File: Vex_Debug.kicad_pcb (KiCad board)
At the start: 2 copper layers, 26 x 54 mm, 31 parts, among them J1 USB_C_Receptacle_USB2.0, U1 ESP32-C3-MINI-1-N4, U2 NCP1117-3.3_SOT223, U3 ADM3493ARZ

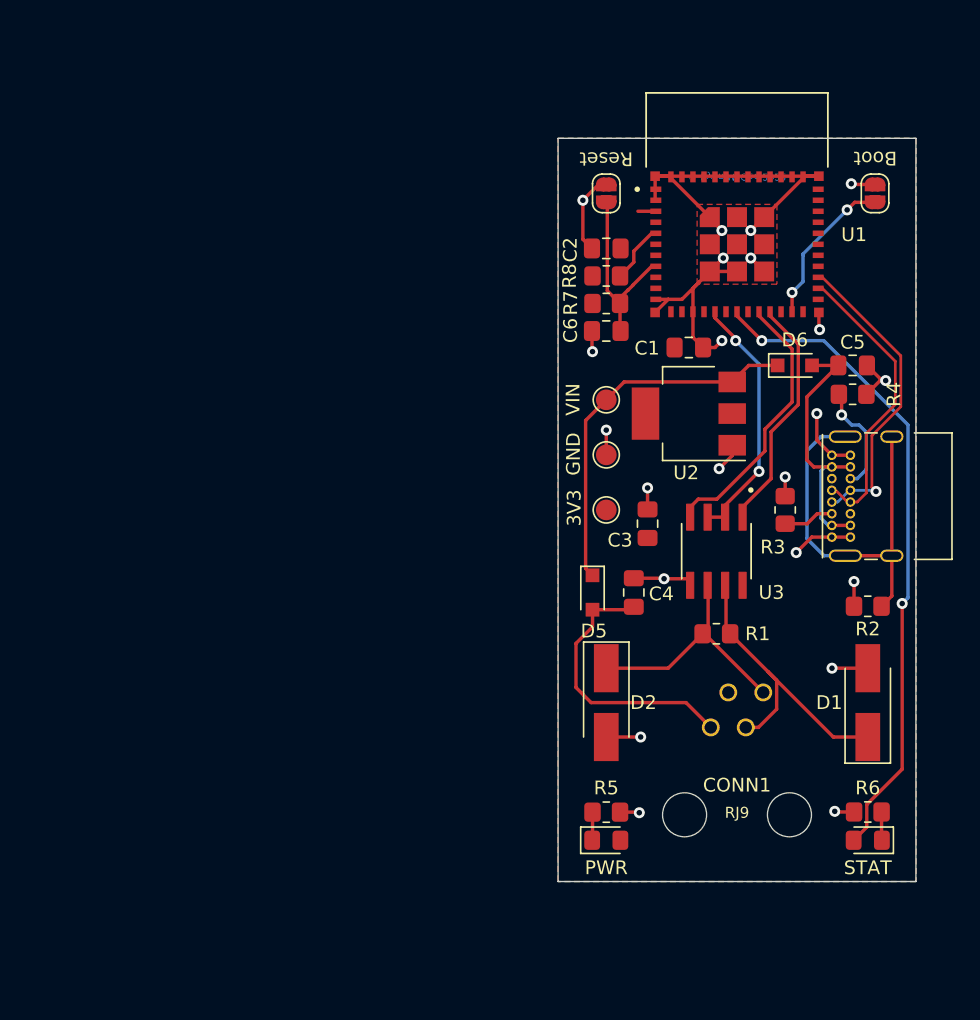
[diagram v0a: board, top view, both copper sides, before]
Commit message: Revision 2.1 release
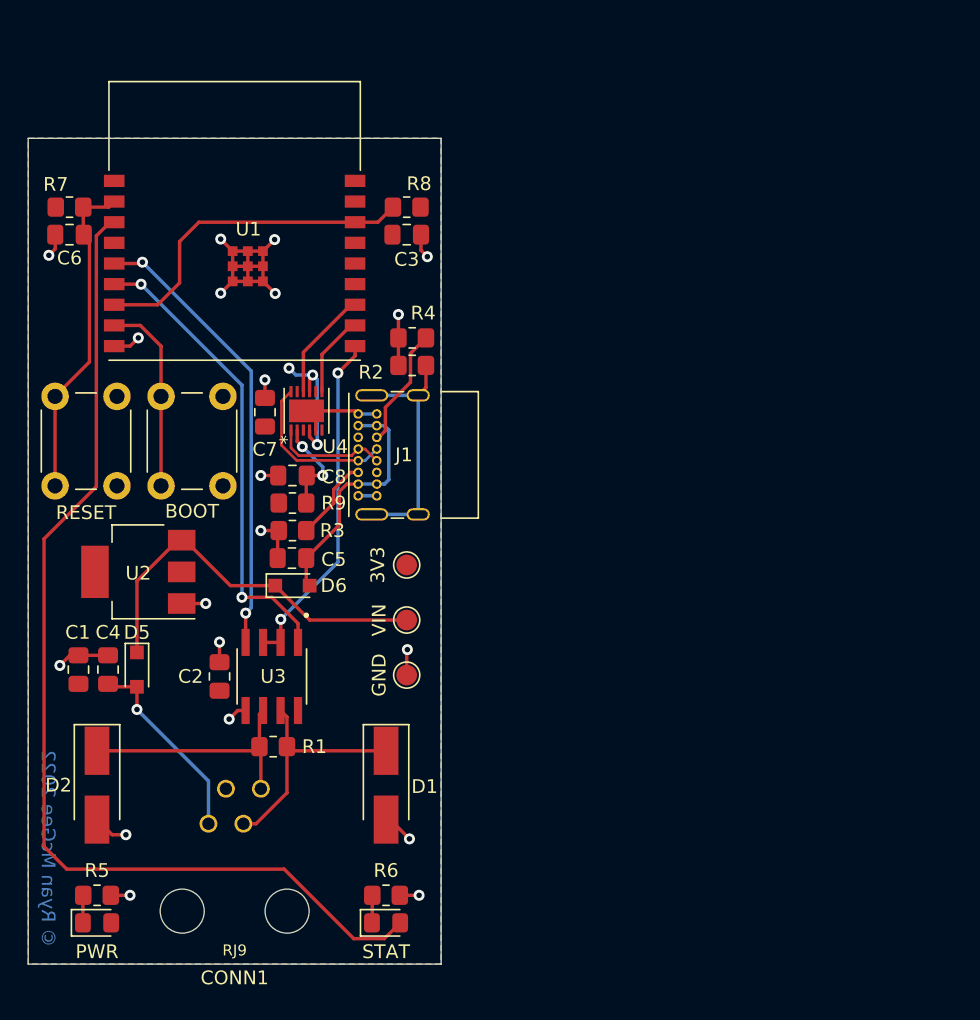
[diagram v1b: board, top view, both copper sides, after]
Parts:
- removed JP1, JP2: SolderJumper_2_Open, Jumper:SolderJumper-2_P1.3mm_Open_RoundedPad1.0x1.5mm
- added C7: 1uF, Capacitor_SMD:C_0805_2012Metric_Pad1.18x1.45mm_HandSolder, F.Cu at (97.2, 79.9)
- added C8: 1uF, Capacitor_SMD:C_0805_2012Metric_Pad1.18x1.45mm_HandSolder, F.Cu at (99.2, 84.5)
- added R9: 5.11K, Resistor_SMD:R_0805_2012Metric_Pad1.20x1.40mm_HandSolder, F.Cu at (99.2, 86.5)
- added SW1: RESET, Button_Switch_THT:SW_PUSH_6mm, F.Cu at (86.5, 78.8)
- added SW2: BOOT, Button_Switch_THT:SW_PUSH_6mm, F.Cu at (94.2, 78.8)
- added U4: FT234XD-R, USB-UART Bridge:FT234XD-R, F.Cu at (100.2, 79.8)
- R7, R8: value 10K -> 5.11K
- U1: value ESP32-C3-MINI-1-N4 -> ESP32-C3-WROOM-02-N4; footprint ESP32-C3-MINI:XCVR_ESP32-C3-MINI-1-N4 -> ESP32-C3-WROOM:ESP32-C3-WROOM-02-N4
- moved C1 50.1 mm to (83.7, 98.6), turned to 90 degrees
- moved G*** 44.7 mm to (94.2, 67.8), turned to 180 degrees
- moved C5 43.1 mm to (99.2, 90.5), turned to 180 degrees
- moved C2 41.9 mm to (93.9, 99.1), turned to 90 degrees
- moved U2 41.6 mm to (88.0, 91.5)
- moved D6 39.9 mm to (99.2, 92.5)
- moved C6 39.6 mm to (83.0, 67.0)
- moved R7 39.6 mm to (83.0, 65.0), turned to 180 degrees
- moved C4 38.6 mm to (85.8, 98.6)
- moved R5 37.5 mm to (85.0, 115.0)
- moved D2 37.5 mm to (85.0, 107.0)
- moved D3 37.5 mm to (85.0, 117.0)
- moved R2 37.4 mm to (107.9, 76.5)
- moved CONN1 37.2 mm to (95.0, 115.0)
- moved U1 36.5 mm to (95.0, 66.0)
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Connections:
- R7 pad 1: +3.3V -> Net-(C6-Pad1)
- R7 pad 2: Net-(C6-Pad1) -> +3.3V
- R8 pad 1: +3.3V -> /IO8_PULLUP
- R8 pad 2: Net-(R8-Pad2) -> +3.3V
- U1 pad 1: GND -> +3.3V
- U1 pad 10: unconnected-(U1-Pad10) -> /RS485_MODE
- U1 pad 11: GND -> /FTDI_TX
- U1 pad 12: unconnected-(U1-Pad12) -> /FTDI_RX
- U1 pad 14: GND -> unconnected-(U1-Pad14)
- U1 pad 16: /RS485_MODE -> /IO8_PULLUP
- U1 pad 18: /STAT_LED -> unconnected-(U1-Pad18)
- U1 pad 19: unconnected-(U1-Pad19) -> GND
- U1 pad 2: GND -> Net-(C6-Pad1)
- U1 pad 20: /RS485_TX -> GND
- U1 pad 21: /RS485_RX -> GND
- U1 pad 22: unconnected-(U1-Pad22) -> GND
- U1 pad 23: Net-(JP2-Pad1) -> GND
- U1 pad 24: unconnected-(U1-Pad24) -> GND
- U1 pad 25: unconnected-(U1-Pad25) -> GND
- U1 pad 26: /USB_D- -> GND
- U1 pad 27: /USB_D+ -> GND
- U1 pad 3: +3.3V -> /STAT_LED
- U1 pad 5: Net-(R8-Pad2) -> /RS485_TX
- U1 pad 6: unconnected-(U1-Pad6) -> /RS485_RX
- U1 pad 7: unconnected-(U1-Pad7) -> /IO8_PULLUP
- U1 pad 8: Net-(C6-Pad1) -> Net-(SW2-Pad2)
- U1 pad 9: unconnected-(U1-Pad9) -> GND
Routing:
- net GND: track 88.8 -> 59.4 mm, vias 22 -> 20
- net /STAT_LED: track 47.8 -> 76.8 mm, vias 2 -> 0
- net /IO8_PULLUP: track 0.00 -> 24.9 mm
- net /RS485_RX: track 17.5 -> 34.0 mm, vias 0 -> 2
- net Net-(SW2-Pad2): track 0.00 -> 14.2 mm
- net /RS485_TX: track 19.8 -> 33.2 mm, vias 0 -> 2
- net /USB_D-: track 21.0 -> 8.31 mm
- net Net-(JP2-Pad1): track 11.3 -> 0.00 mm, vias 2 -> 0
- net Net-(J1-PadS1): track 28.9 -> 17.8 mm
- net /USB_D+: track 22.8 -> 11.9 mm, vias 1 -> 0
- net Net-(C6-Pad1): track 13.7 -> 23.9 mm
- net +3.3V: track 1.30 -> 9.69 mm, vias 0 -> 3
- net /FTDI_RX: track 0.00 -> 8.04 mm
- net Net-(C8-Pad1): track 0.00 -> 7.25 mm, vias 0 -> 2
- net /RS485_MODE: track 18.5 -> 25.0 mm
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- removed copper zone on F.Cu, net GND
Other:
- board size 26 x 54 mm -> 30 x 60 mm
- board text added: "V5 Debug Board 11/27/2022 Rev 2.1"
- board text removed: "V5 Debug Board 10/23/2022 Rev 1"

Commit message: Updated to revision 3.0
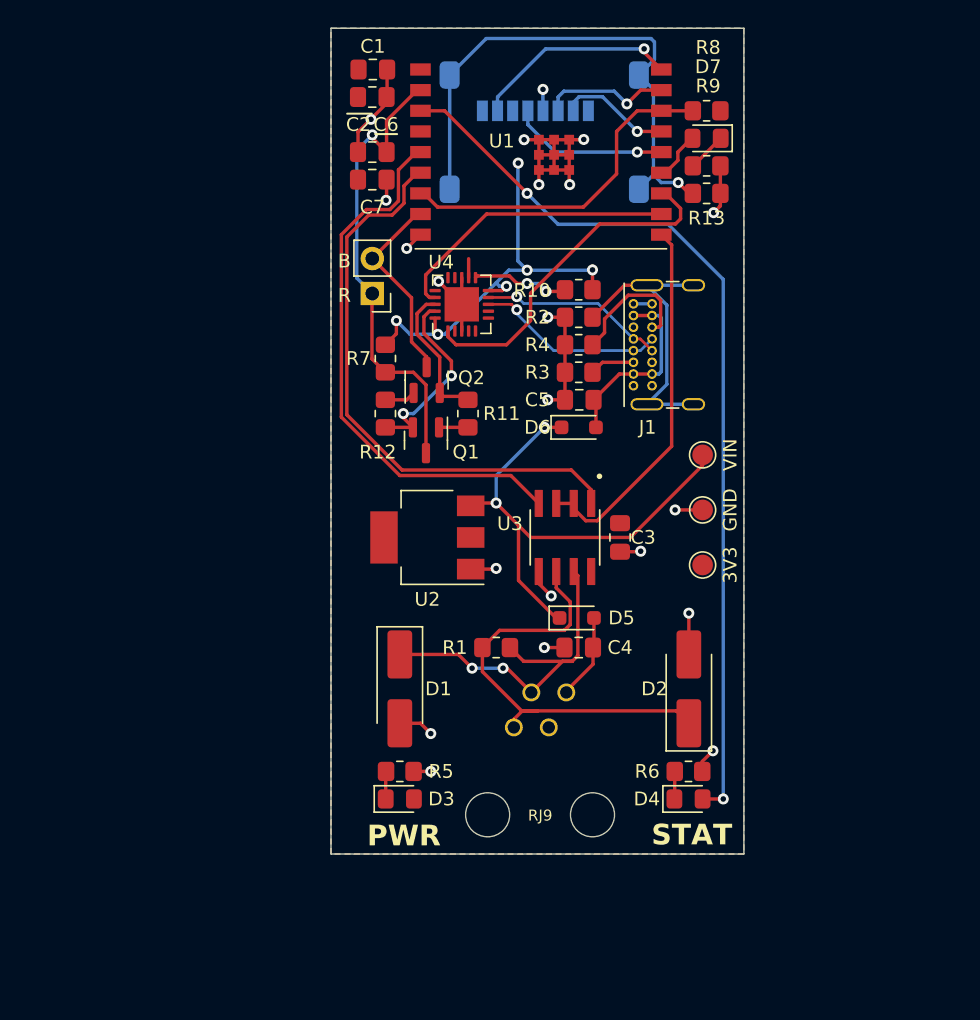
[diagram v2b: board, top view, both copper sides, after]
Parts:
- removed C8: 1uF, Capacitor_SMD:C_0805_2012Metric_Pad1.18x1.45mm_HandSolder
- removed SW1: RESET, Button_Switch_THT:SW_PUSH_6mm
- removed SW2: BOOT, Button_Switch_THT:SW_PUSH_6mm
- removed TP1: TP_VIN, TestPoint:TestPoint_Pad_D1.5mm
- removed TP2: TP_GND, TestPoint:TestPoint_Pad_D1.5mm
- removed TP3: TP_3.3V, TestPoint:TestPoint_Pad_D1.5mm
- added 3V3: TP_3.3V, TestPoint:TestPoint_Pad_D1.5mm, F.Cu at (129.0, 91.0)
- added D7: DBG_LED, LED_SMD:LED_0805_2012Metric_Pad1.15x1.40mm_HandSolder, F.Cu at (129.3, 60.0)
- added GND: TP_GND, TestPoint:TestPoint_Pad_D1.5mm, F.Cu at (129.0, 87.0)
- added J2: Micro_SD_Card, Connector_Card:microSD_HC_Molex_47219-2001, B.Cu at (117.5, 60.1)
- added J3: Conn_01x02_Pin, Connector_PinHeader_2.54mm:PinHeader_1x02_P2.54mm_Vertical, F.Cu at (105.0, 71.3)
- added Q1: BC817, Package_TO_SOT_SMD:SOT-23, F.Cu at (108.9, 81.9)
- added Q2: BC817, Package_TO_SOT_SMD:SOT-23, F.Cu at (109.0, 77.6)
- added R10: 5.11K, Resistor_SMD:R_0805_2012Metric_Pad1.20x1.40mm_HandSolder, F.Cu at (120.0, 71.0)
- added R11: 5.11K, Resistor_SMD:R_0805_2012Metric_Pad1.20x1.40mm_HandSolder, F.Cu at (112.0, 80.0)
- added R12: 5.11K, Resistor_SMD:R_0805_2012Metric_Pad1.20x1.40mm_HandSolder, F.Cu at (106.0, 80.0)
- added R13: 1M, Resistor_SMD:R_0805_2012Metric_Pad1.20x1.40mm_HandSolder, F.Cu at (129.3, 64.0)
- added VIN: TP_VIN, TestPoint:TestPoint_Pad_D1.5mm, F.Cu at (129.0, 83.0)
- R9: value 5.11K -> 220
- U4: value FT234XD-R -> FT231XQ; footprint USB-UART Bridge:FT234XD-R -> Package_DFN_QFN:QFN-20-1EP_4x4mm_P0.5mm_EP2.5x2.5mm
- moved C1 48.6 mm to (105.0, 55.0), turned to 0 degrees
- moved D2 43.6 mm to (128.0, 100.0), turned to 90 degrees
- moved C2 43.5 mm to (105.0, 57.0), turned to 0 degrees
- moved R9 38.8 mm to (129.3, 62.0), turned to 0 degrees
- moved C4 34.2 mm to (120.0, 97.0), turned to 180 degrees
- moved D5 32.2 mm to (119.9, 94.8), turned to 0 degrees
- moved G*** 29.9 mm to (116.1, 88.2)
- moved C3 26.9 mm to (123.0, 89.0), turned to -90 degrees
- moved R7 25.4 mm to (106.0, 76.0), turned to 90 degrees
- moved C5 23.8 mm to (120.0, 79.0)
- moved D3 23.8 mm to (107.0, 108.0)
- moved R5 23.8 mm to (107.0, 106.0)
- moved D6 23.8 mm to (120.0, 81.0)
- moved R3 23.8 mm to (120.0, 77.0)
- moved D4 23.7 mm to (128.0, 108.0)
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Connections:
- net Net-(C6-Pad1) renamed /EN_PU
- C4 pad 1: Net-(C4-Pad1) -> Net-(CONN1-+12V)
- CONN1 pad 1: Net-(C4-Pad1) -> /RJ9_DA
- CONN1 pad 2: GND -> /RJ9_DB
- CONN1 pad 3: /RJ9_DB -> GND
- CONN1 pad 4: /RJ9_DA -> Net-(CONN1-+12V)
- D5 pad 2: Net-(C4-Pad1) -> Net-(CONN1-+12V)
- R9 pad 1: Net-(C8-Pad1) -> Net-(D7-K)
- R9 pad 2: +3.3V -> GND
- U1 pad 13: unconnected-(U1-Pad13) -> /DBG_LED
- U1 pad 14: unconnected-(U1-Pad14) -> /SD_SCL
- U1 pad 15: unconnected-(U1-Pad15) -> /SD_CS
- U1 pad 17: unconnected-(U1-Pad17) -> /SD_MOSI
- U1 pad 18: unconnected-(U1-Pad18) -> /SD_MISO
- U1 pad 8: Net-(SW2-Pad2) -> /IO9_BOOT
- U4 pad 1: /USB_D- -> /FTDI_RX
- U4 pad 10: /FTDI_RX -> +3.3V
- U4 pad 11: unconnected-(U4-Pad11) -> Net-(U4-~{RESET})
- U4 pad 12: /USB_D+ -> +3.3V
- U4 pad 2: Net-(C8-Pad1) -> unconnected-(U4-~{RI}-Pad2)
- U4 pad 3: unconnected-(U4-Pad3) -> GND
- U4 pad 4: +3.3V -> unconnected-(U4-~{DSR}-Pad4)
- U4 pad 5: GND -> unconnected-(U4-~{DCD}-Pad5)
- U4 pad 7: /FTDI_TX -> unconnected-(U4-CBUS2-Pad7)
- U4 pad 8: unconnected-(U4-Pad8) -> /USB_D+
- U4 pad 9: +3.3V -> /USB_D-
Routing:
- net Net-(J2-SHIELD): track 0.00 -> 40.8 mm, vias 0 -> 1
- net +3.3V: track 9.69 -> 34.8 mm, vias 3 -> 7
- net /FTDI_RX: track 8.04 -> 25.1 mm
- net /FTDI_TX: track 5.98 -> 21.1 mm
- net /SD_MISO: track 0.00 -> 15.1 mm, vias 0 -> 1
- net /RJ9_DA: track 17.8 -> 32.2 mm
- net /IO9_BOOT: track 0.00 -> 14.4 mm
- net Net-(C4-Pad1): track 14.3 -> 0.00 mm, vias 1 -> 0
- net Net-(SW2-Pad2): track 14.2 -> 0.00 mm
- net Net-(Q1-E): track 0.00 -> 14.0 mm, vias 0 -> 2
- net /SD_SCL: track 0.00 -> 11.5 mm, vias 0 -> 1
- net /STAT_LED: track 76.8 -> 66.3 mm, vias 0 -> 2
- net /EN_PU: track 23.9 -> 34.2 mm, vias 0 -> 1
- net Net-(Q2-E): track 0.00 -> 10.3 mm
- net /SD_MOSI: track 0.00 -> 9.47 mm, vias 0 -> 1
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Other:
- board text added: "- C7 decoupler to FTDI chip - Rotate decoupling caps for shortest path to 3v3 - UART TX/RX too close - FTDI RTS/DTR may be inverted? :("
- board text added: "B"
- board text added: "PWR"
- board text added: "R"
- board text added: "STAT"
- board text added: "V5 Debug Board Rev 3.0 12/30/2023"
- board text removed: "V5 Debug Board 11/27/2022 Rev 2.1"
- board text removed: "© Ryan McGee 2022"
